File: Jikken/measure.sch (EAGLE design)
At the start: 4 parts

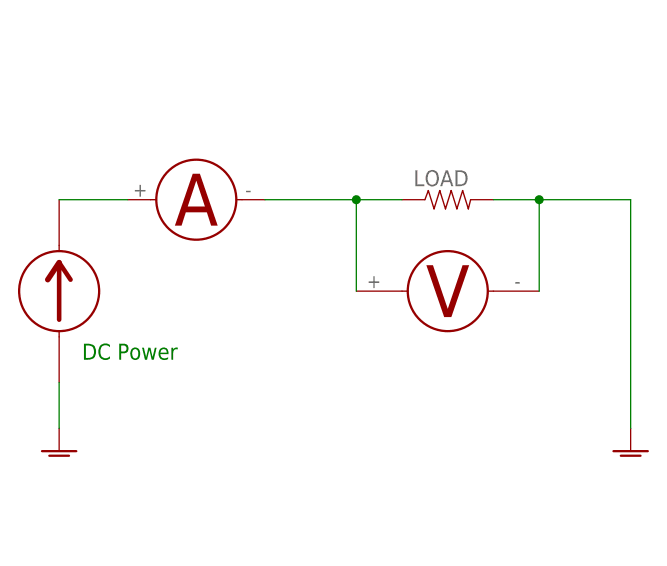
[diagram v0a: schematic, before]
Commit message: mylib
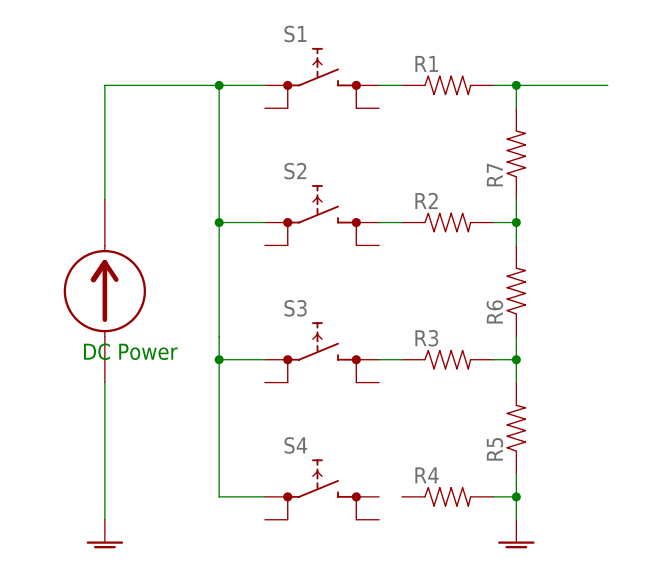
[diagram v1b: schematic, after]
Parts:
- removed LOAD: (no value), My Library:RESISTORPTH-1/4W
- removed U$1: AMMETER, My Library:AMMETER
- removed U$2: VOLTMETER, My Library:VOLTMETER
- added R1, R2, R3, R4, R5, R6, R7: (no value), My Library:RESISTORPTH-1/4W
- added S1, S2, S3, S4: (no value), switch:REKN
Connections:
- new net N$3: R2.1, S2.1@A
- new net N$4: R3.1, S3.1@A
- new net N$5: R1.2, R7.2
- new net N$6: R2.2, R6.2, R7.1
- new net N$7: R3.2, R5.2, R6.1
- net AGND: now also R4.2, R5.1; no longer LOAD.2, U$2.P$2
- net N$1: now also S1.0@A, S2.0@A, S3.0@A, S4.0@A; no longer U$1.P$1
- net N$2: now also R1.1, S1.1@A; no longer LOAD.1, U$1.P$2, U$2.P$1
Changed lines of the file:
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@@
 </classes>
 <parts>
-<part name="U$1" library="My Library" deviceset="AMMETER" device=""/>
-<part name="U$2" library="My Library" deviceset="VOLTMETER" device=""/>
-<part name="LOAD" library="My Library" deviceset="RESISTOR" device="PTH-1/4W"/>
+<part name="R2" library="My Library" deviceset="RESISTOR" device="PTH-1/4W"/>
 <part name="DC_POEWR" library="My Library" deviceset="DCPOWER" device=""/>
 <part name="SUPPLY1" library="supply1" deviceset="AGND" device=""/>
 <part name="SUPPLY2" library="supply1" deviceset="AGND" device=""/>
+<part name="R1" library="My Library" deviceset="RESISTOR" device="PTH-1/4W"/>
+<part name="R3" library="My Library" deviceset="RESISTOR" device="PTH-1/4W"/>
+<part name="R4" library="My Library" deviceset="RESISTOR" device="PTH-1/4W"/>
+<part name="R5" library="My Library" deviceset="RESISTOR" device="PTH-1/4W"/>
+<part name="R6" library="My Library" deviceset="RESISTOR" device="PTH-1/4W"/>
+<part name="R7" library="My Library" deviceset="RESISTOR" device="PTH-1/4W"/>
+<part name="S1" library="switch" deviceset="REKN" device=""/>
+<part name="S2" library="switch" deviceset="REKN" device=""/>
+<part name="S3" library="switch" deviceset="REKN" device=""/>
+<part name="S4" library="switch" deviceset="REKN" device=""/>
 </parts>
 <sheets>
@@
 </plain>
 <instances>
-<instance part="U$1" gate="G$1" x="63.5" y="66.04"/>
-<instance part="U$2" gate="G$1" x="91.44" y="55.88"/>
-<instance part="LOAD" gate="G$1" x="91.44" y="66.04"/>
-<instance part="DC_POEWR" gate="G$1" x="48.26" y="55.88"/>
-<instance part="SUPPLY1" gate="VR1" x="48.26" y="38.1" smashed="yes"/>
-<instance part="SUPPLY2" gate="VR1" x="111.76" y="38.1" smashed="yes"/>
+<instance part="R2" gate="G$1" x="91.44" y="63.5"/>
+<instance part="DC_POEWR" gate="G$1" x="53.34" y="55.88"/>
+<instance part="SUPPLY1" gate="VR1" x="53.34" y="27.94" smashed="yes"/>
+<instance part="SUPPLY2" gate="VR1" x="99.06" y="27.94" smashed="yes"/>
+<instance part="R1" gate="G$1" x="91.44" y="78.74"/>
+<instance part="R3" gate="G$1" x="91.44" y="48.26"/>
+<instance part="R4" gate="G$1" x="91.44" y="33.02"/>
+<instance part="R5" gate="G$1" x="99.06" y="40.64" rot="R90"/>
+<instance part="R6" gate="G$1" x="99.06" y="55.88" rot="R90"/>
+<instance part="R7" gate="G$1" x="99.06" y="71.12" rot="R90"/>
+<instance part="S1" gate="G$1" x="76.2" y="78.74"/>
+<instance part="S2" gate="G$1" x="76.2" y="63.5"/>
+<instance part="S3" gate="G$1" x="76.2" y="48.26"/>
+<instance part="S4" gate="G$1" x="76.2" y="33.02"/>
 </instances>
 <busses>
@@
 <net name="N$1" class="0">
 <segment>
-<pinref part="U$1" gate="G$1" pin="P$1"/>
-<wire x1="48.26" y1="66.04" x2="55.88" y2="66.04" width="0.1524" layer="91"/>
+<wire x1="53.34" y1="66.04" x2="53.34" y2="78.74" width="0.1524" layer="91"/>
+<wire x1="53.34" y1="78.74" x2="66.04" y2="78.74" width="0.1524" layer="91"/>
 <pinref part="DC_POEWR" gate="G$1" pin="VOUT"/>
-</segment>
-</net>
-<net name="N$2" class="0">
-<segment>
-<pinref part="U$1" gate="G$1" pin="P$2"/>
-<pinref part="LOAD" gate="G$1" pin="1"/>
-<wire x1="71.12" y1="66.04" x2="81.28" y2="66.04" width="0.1524" layer="91"/>
-<pinref part="U$2" gate="G$1" pin="P$1"/>
-<wire x1="81.28" y1="66.04" x2="86.36" y2="66.04" width="0.1524" layer="91"/>
-<wire x1="81.28" y1="55.88" x2="81.28" y2="66.04" width="0.1524" layer="91"/>
-<junction x="81.28" y="66.04"/>
+<pinref part="S1" gate="G$1" pin="0@A"/>
+<wire x1="66.04" y1="78.74" x2="71.12" y2="78.74" width="0.1524" layer="91"/>
+<wire x1="66.04" y1="78.74" x2="66.04" y2="63.5" width="0.1524" layer="91"/>
+<pinref part="S4" gate="G$1" pin="0@A"/>
+<wire x1="66.04" y1="63.5" x2="66.04" y2="50.8" width="0.1524" layer="91"/>
+<wire x1="66.04" y1="48.26" x2="66.04" y2="33.02" width="0.1524" layer="91"/>
+<wire x1="66.04" y1="33.02" x2="71.12" y2="33.02" width="0.1524" layer="91"/>
+<pinref part="S3" gate="G$1" pin="0@A"/>
+<wire x1="71.12" y1="48.26" x2="66.04" y2="48.26" width="0.1524" layer="91"/>
+<wire x1="66.04" y1="48.26" x2="66.04" y2="50.8" width="0.1524" layer="91"/>
+<pinref part="S2" gate="G$1" pin="0@A"/>
+<wire x1="71.12" y1="63.5" x2="66.04" y2="63.5" width="0.1524" layer="91"/>
+<junction x="66.04" y="48.26"/>
+<junction x="66.04" y="63.5"/>
+<junction x="66.04" y="78.74"/>
 </segment>
 </net>
@@
 <segment>
 <pinref part="DC_POEWR" gate="G$1" pin="VGND"/>
-<wire x1="48.26" y1="45.72" x2="48.26" y2="40.64" width="0.1524" layer="91"/>
+<wire x1="53.34" y1="45.72" x2="53.34" y2="30.48" width="0.1524" layer="91"/>
 <pinref part="SUPPLY1" gate="VR1" pin="AGND"/>
 </segment>
 <segment>
-<pinref part="LOAD" gate="G$1" pin="2"/>
-<wire x1="96.52" y1="66.04" x2="101.6" y2="66.04" width="0.1524" layer="91"/>
-<wire x1="101.6" y1="66.04" x2="111.76" y2="66.04" width="0.1524" layer="91"/>
-<wire x1="111.76" y1="66.04" x2="111.76" y2="40.64" width="0.1524" layer="91"/>
-<pinref part="U$2" gate="G$1" pin="P$2"/>
-<wire x1="101.6" y1="55.88" x2="101.6" y2="66.04" width="0.1524" layer="91"/>
+<pinref part="R5" gate="G$1" pin="1"/>
+<wire x1="99.06" y1="35.56" x2="99.06" y2="33.02" width="0.1524" layer="91"/>
+<pinref part="R4" gate="G$1" pin="2"/>
+<wire x1="99.06" y1="33.02" x2="96.52" y2="33.02" width="0.1524" layer="91"/>
 <pinref part="SUPPLY2" gate="VR1" pin="AGND"/>
-<junction x="101.6" y="66.04"/>
+<wire x1="99.06" y1="30.48" x2="99.06" y2="33.02" width="0.1524" layer="91"/>
+<junction x="99.06" y="33.02"/>
 </segment>
 </net>
+<net name="N$2" class="0">
+<segment>
+<pinref part="S1" gate="G$1" pin="1@A"/>
+<pinref part="R1" gate="G$1" pin="1"/>
+<wire x1="83.82" y1="78.74" x2="86.36" y2="78.74" width="0.1524" layer="91"/>
+</segment>
+</net>
+<net name="N$3" class="0">
+<segment>
+<pinref part="S2" gate="G$1" pin="1@A"/>
+<pinref part="R2" gate="G$1" pin="1"/>
+<wire x1="83.82" y1="63.5" x2="86.36" y2="63.5" width="0.1524" layer="91"/>
+</segment>
+</net>
+<net name="N$4" class="0">
+<segment>
+<pinref part="S3" gate="G$1" pin="1@A"/>
+<pinref part="R3" gate="G$1" pin="1"/>
+<wire x1="83.82" y1="48.26" x2="86.36" y2="48.26" width="0.1524" layer="91"/>
+</segment>
+</net>
+<net name="N$5" class="0">
+<segment>
+<pinref part="R1" gate="G$1" pin="2"/>
+<pinref part="R7" gate="G$1" pin="2"/>
+<wire x1="96.52" y1="78.74" x2="99.06" y2="78.74" width="0.1524" layer="91"/>
+<wire x1="99.06" y1="78.74" x2="99.06" y2="76.2" width="0.1524" layer="91"/>
+<wire x1="99.06" y1="78.74" x2="109.22" y2="78.74" width="0.1524" layer="91"/>
+<junction x="99.06" y="78.74"/>
+</segment>
+</net>
+<net name="N$6" class="0">
+<segment>
+<pinref part="R7" gate="G$1" pin="1"/>
+<wire x1="99.06" y1="66.04" x2="99.06" y2="63.5" width="0.1524" layer="91"/>
+<pinref part="R2" gate="G$1" pin="2"/>
+<wire x1="99.06" y1="63.5" x2="96.52" y2="63.5" width="0.1524" layer="91"/>
+<pinref part="R6" gate="G$1" pin="2"/>
+<wire x1="99.06" y1="63.5" x2="99.06" y2="60.96" width="0.1524" layer="91"/>
+<junction x="99.06" y="63.5"/>
+</segment>
+</net>
+<net name="N$7" class="0">
+<segment>
+<pinref part="R6" gate="G$1" pin="1"/>
+<wire x1="99.06" y1="50.8" x2="99.06" y2="48.26" width="0.1524" layer="91"/>
+<pinref part="R3" gate="G$1" pin="2"/>
+<wire x1="99.06" y1="48.26" x2="96.52" y2="48.26" width="0.1524" layer="91"/>
+<pinref part="R5" gate="G$1" pin="2"/>
+<wire x1="99.06" y1="48.26" x2="99.06" y2="45.72" width="0.1524" layer="91"/>
+<junction x="99.06" y="48.26"/>
+</segment>
+</net>
